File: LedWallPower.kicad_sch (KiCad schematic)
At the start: 33 parts, among them U201 TPS5430DDA

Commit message: Change LCSC partnumbers for LEDS and NM for testpoints
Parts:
- TP201, TP202, TP203, TP204, TP205, TP206, TP207, TP208, TP209, TP210, TP211, TP212, TP213, TP214, TP215, TP216, TP217, TP218: LCSC C238122 -> (none)
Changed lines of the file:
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@@
       (effects (font (size 1.27 1.27)) hide)
     )
-    (property "LCSC" "C238122" (id 4) (at 135.89 63.5 0)
+    (property "LCSC" "" (id 4) (at 135.89 63.5 0)
       (effects (font (size 1.27 1.27)) hide)
     )
@@
       (effects (font (size 1.27 1.27)) hide)
     )
-    (property "LCSC" "C238122" (id 4) (at 124.46 175.26 0)
+    (property "LCSC" "" (id 4) (at 124.46 175.26 0)
       (effects (font (size 1.27 1.27)) hide)
     )
@@
       (effects (font (size 1.27 1.27)) hide)
     )
-    (property "LCSC" "C238122" (id 4) (at 111.76 175.26 0)
+    (property "LCSC" "" (id 4) (at 111.76 175.26 0)
       (effects (font (size 1.27 1.27)) hide)
     )
@@
       (effects (font (size 1.27 1.27)) hide)
     )
-    (property "LCSC" "C238122" (id 4) (at 182.88 44.45 0)
+    (property "LCSC" "" (id 4) (at 182.88 44.45 0)
       (effects (font (size 1.27 1.27)) hide)
     )
@@
       (effects (font (size 1.27 1.27)) hide)
     )
-    (property "LCSC" "C238122" (id 4) (at 137.16 175.26 0)
+    (property "LCSC" "" (id 4) (at 137.16 175.26 0)
       (effects (font (size 1.27 1.27)) hide)
     )
@@
       (effects (font (size 1.27 1.27)) hide)
     )
-    (property "LCSC" "C238122" (id 4) (at 99.06 175.26 0)
+    (property "LCSC" "" (id 4) (at 99.06 175.26 0)
       (effects (font (size 1.27 1.27)) hide)
     )
@@
       (effects (font (size 1.27 1.27)) hide)
     )
-    (property "LCSC" "C238122" (id 4) (at 81.28 53.34 0)
+    (property "LCSC" "" (id 4) (at 81.28 53.34 0)
       (effects (font (size 1.27 1.27)) hide)
     )
@@
       (effects (font (size 1.27 1.27)) hide)
     )
-    (property "LCSC" "C238122" (id 4) (at 99.06 187.96 0)
+    (property "LCSC" "" (id 4) (at 99.06 187.96 0)
       (effects (font (size 1.27 1.27)) hide)
     )
@@
       (effects (font (size 1.27 1.27)) hide)
     )
-    (property "LCSC" "C238122" (id 4) (at 217.17 44.45 0)
+    (property "LCSC" "" (id 4) (at 217.17 44.45 0)
       (effects (font (size 1.27 1.27)) hide)
     )
@@
       (effects (font (size 1.27 1.27)) hide)
     )
-    (property "LCSC" "C238122" (id 4) (at 137.16 187.96 0)
+    (property "LCSC" "" (id 4) (at 137.16 187.96 0)
       (effects (font (size 1.27 1.27)) hide)
     )
@@
       (effects (font (size 1.27 1.27)) hide)
     )
-    (property "LCSC" "C238122" (id 4) (at 124.46 187.96 0)
+    (property "LCSC" "" (id 4) (at 124.46 187.96 0)
       (effects (font (size 1.27 1.27)) hide)
     )
@@
       (effects (font (size 1.27 1.27)) hide)
     )
-    (property "LCSC" "C238122" (id 4) (at 135.89 73.66 0)
+    (property "LCSC" "" (id 4) (at 135.89 73.66 0)
       (effects (font (size 1.27 1.27)) hide)
     )
@@
       (effects (font (size 1.27 1.27)) hide)
     )
-    (property "LCSC" "C238122" (id 4) (at 81.28 73.66 0)
+    (property "LCSC" "" (id 4) (at 81.28 73.66 0)
       (effects (font (size 1.27 1.27)) hide)
     )
@@
       (effects (font (size 1.27 1.27)) hide)
     )
-    (property "LCSC" "C238122" (id 4) (at 149.86 175.26 0)
+    (property "LCSC" "" (id 4) (at 149.86 175.26 0)
       (effects (font (size 1.27 1.27)) hide)
     )
@@
       (effects (font (size 1.27 1.27)) hide)
     )
-    (property "LCSC" "C238122" (id 4) (at 199.39 77.47 0)
+    (property "LCSC" "" (id 4) (at 199.39 77.47 0)
       (effects (font (size 1.27 1.27)) hide)
     )
@@
       (effects (font (size 1.27 1.27)) hide)
     )
-    (property "LCSC" "C238122" (id 4) (at 149.86 187.96 0)
+    (property "LCSC" "" (id 4) (at 149.86 187.96 0)
       (effects (font (size 1.27 1.27)) hide)
     )
@@
       (effects (font (size 1.27 1.27)) hide)
     )
-    (property "LCSC" "C238122" (id 4) (at 182.88 77.47 0)
+    (property "LCSC" "" (id 4) (at 182.88 77.47 0)
       (effects (font (size 1.27 1.27)) hide)
     )
@@
       (effects (font (size 1.27 1.27)) hide)
     )
-    (property "LCSC" "C238122" (id 4) (at 111.76 187.96 0)
-      (effects (font (size 1.27 1.27)) hide)
-    )
+    (property "LCSC" "" (id 4) (at 111.76 187.96 0)
+      (effects (font (size 1.27 1.27)) hide)
+    )

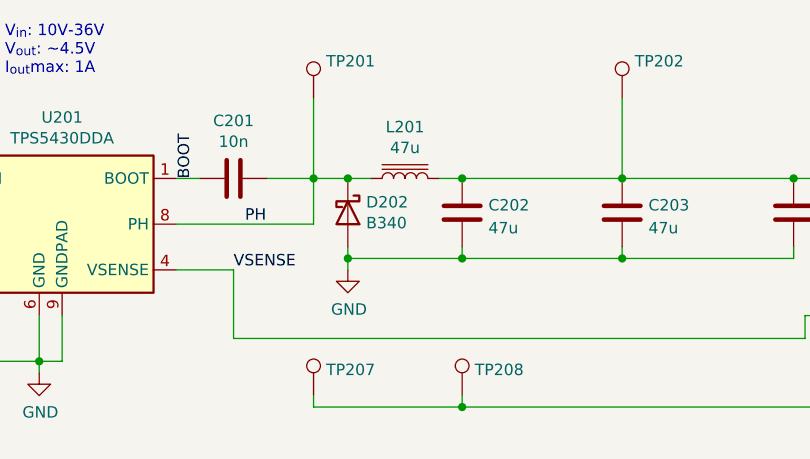
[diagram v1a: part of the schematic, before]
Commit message: Fix small changed for rev2
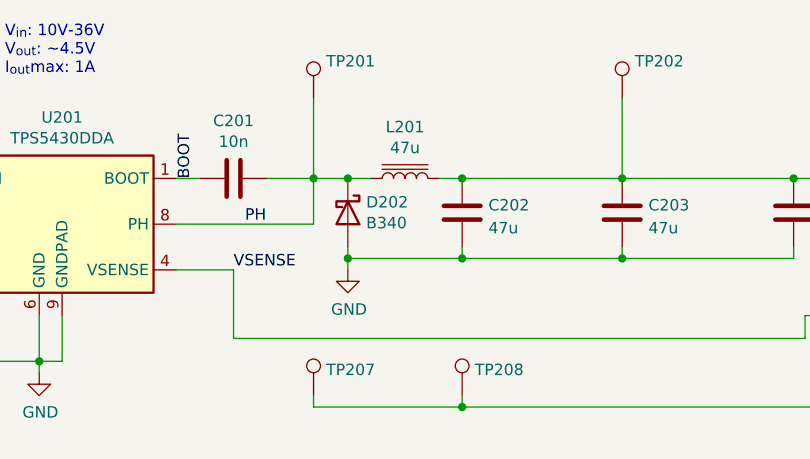
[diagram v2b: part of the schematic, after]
